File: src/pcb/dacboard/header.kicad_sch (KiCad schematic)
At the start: 1 part, among them J4 Conn_01x24_Socket

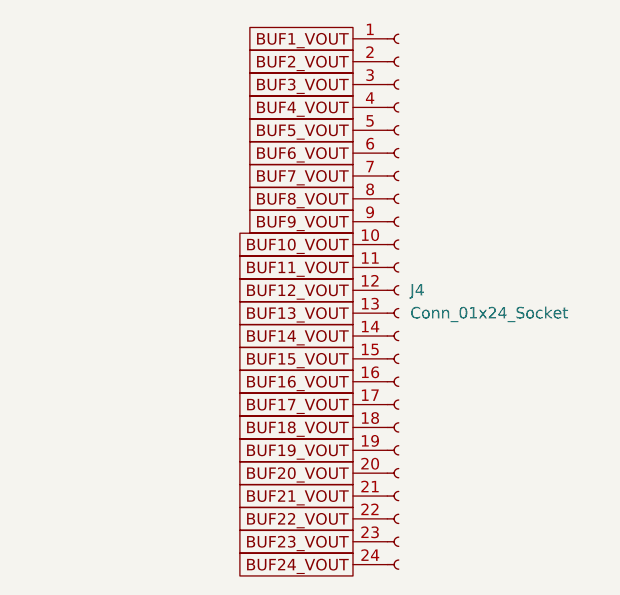
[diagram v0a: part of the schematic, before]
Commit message: dacboard routing
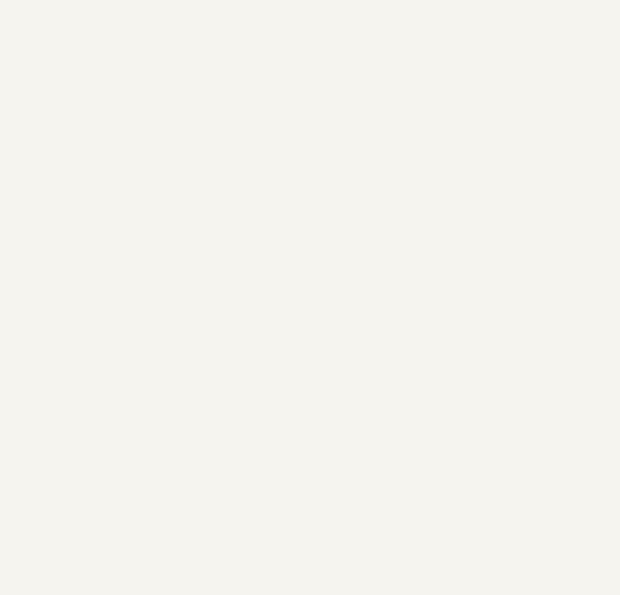
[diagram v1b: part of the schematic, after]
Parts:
- removed J4: Conn_01x24_Socket, symbol Connector:Conn_01x24_Socket
